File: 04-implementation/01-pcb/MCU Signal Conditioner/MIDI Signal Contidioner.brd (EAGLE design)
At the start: 81.3 x 38.1 mm, 15 parts, among them J2 ARDUINO-CONN-8X2, J3 ARDUINO-CONN-8X2, U4 24CS01, U6 MCP1700-SOT89, X1 SSW-107-02-S-D, X2 SSW-107-02-S-D, X3 SSW-107-02-S-D, X4 SSW-107-02-S-D, X5 MINI-USB-SHIELD-32005-201

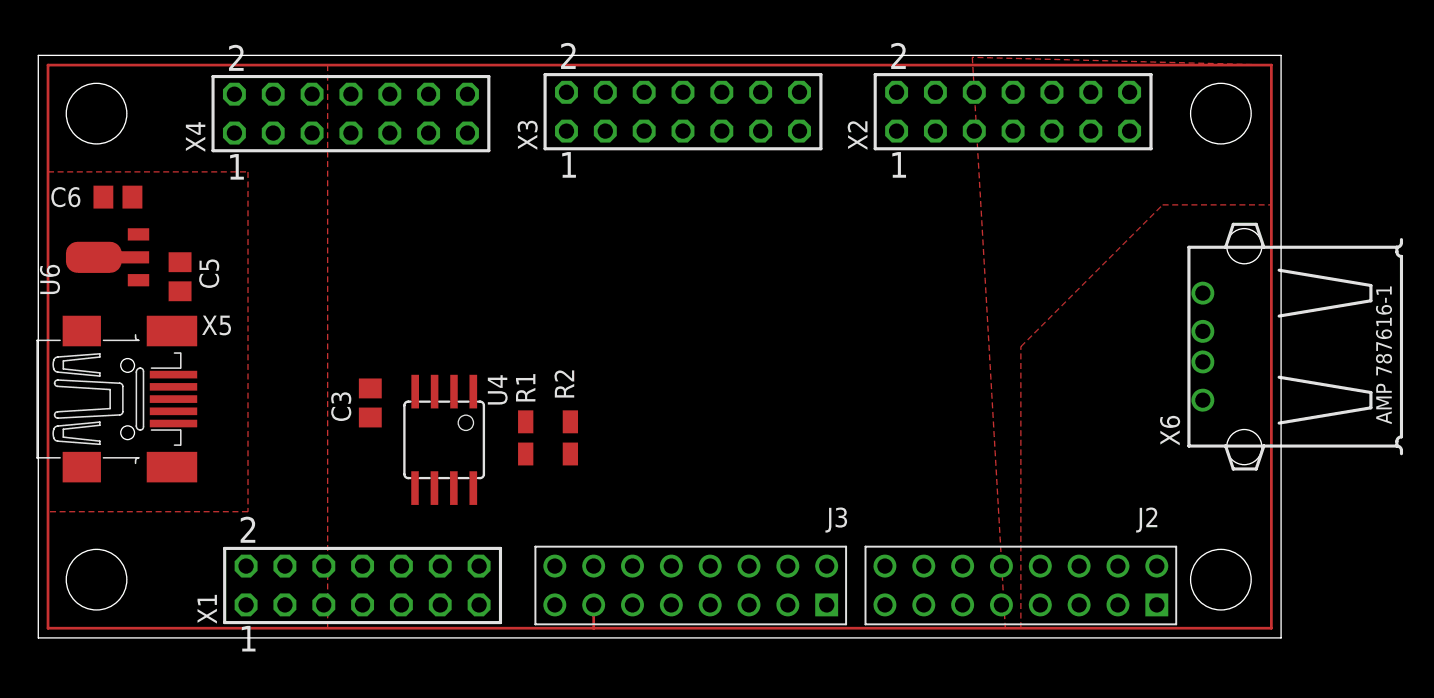
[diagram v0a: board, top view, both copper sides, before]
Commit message: Complete initial placement of components.
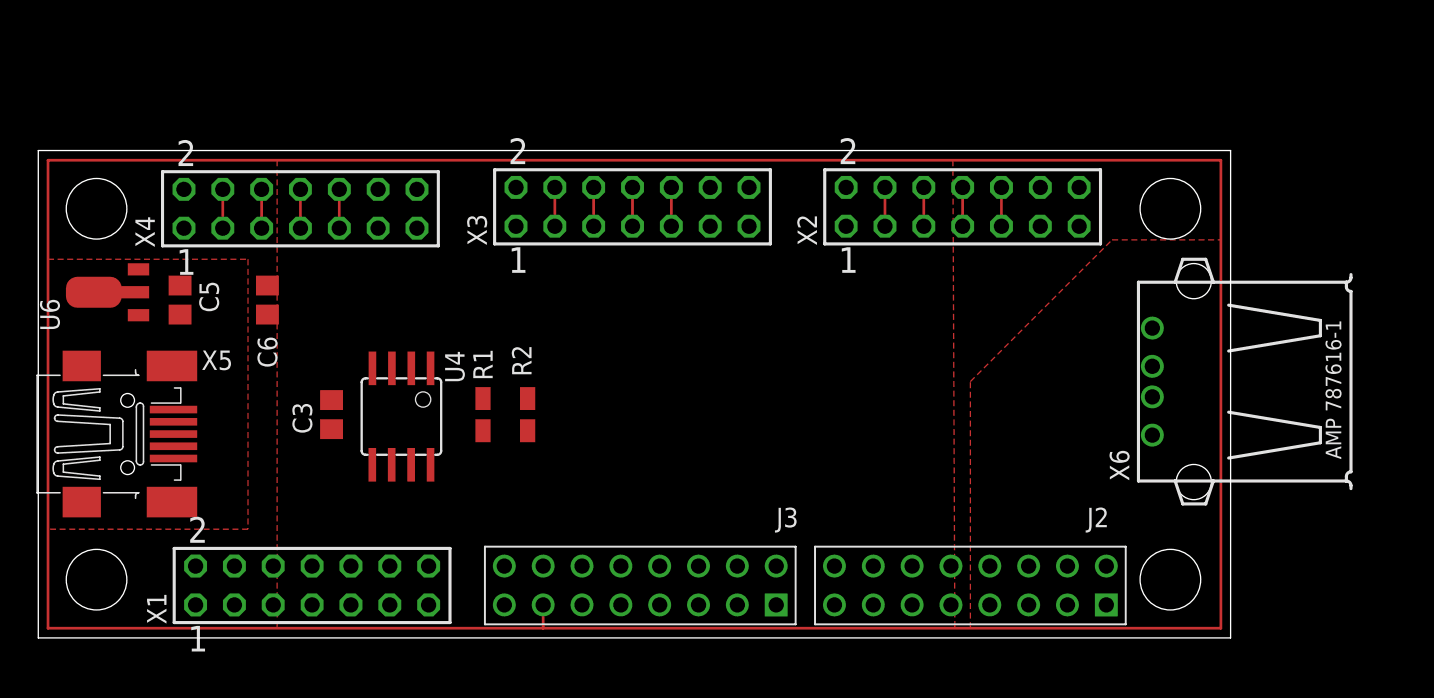
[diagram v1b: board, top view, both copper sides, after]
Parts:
- moved C6 11.9 mm to (15.0, 22.1), turned to 270 degrees
- moved X2 7.04 mm to (60.5, 28.2)
- moved X3 7.04 mm to (38.9, 28.2)
- moved X4 7.04 mm to (17.1, 28.1)
- moved X6 4.02 mm to (85.9, 16.8)
- moved J2 3.30 mm to (69.8, 2.16)
- moved J3 3.30 mm to (48.3, 2.16)
- moved X1 3.30 mm to (17.9, 3.43)
- moved R2 3.18 mm to (32.0, 14.6)
- moved R1 3.18 mm to (29.1, 14.6)
- moved U4 3.18 mm to (23.7, 14.5)
- moved C3 2.65 mm to (19.2, 14.6)
- moved X5 2.29 mm to (5.84, 13.3)
- moved U6 2.29 mm to (4.57, 22.6)
- moved C5 1.52 mm to (9.27, 22.1)
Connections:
- net GND: now also X5.M1, X5.M2, X5.M3, X5.M4
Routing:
- net +5V: track 235.2 -> 216.2 mm
- net DI4: track 0.00 -> 5.08 mm
- net DI3: track 0.00 -> 5.08 mm
- net DI2: track 0.00 -> 5.08 mm
- net DI1: track 0.00 -> 5.08 mm
- net DO4: track 0.00 -> 2.54 mm
- net DO3: track 0.00 -> 2.54 mm
- net DO2: track 0.00 -> 2.54 mm
- net DO1: track 0.00 -> 2.54 mm
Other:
- board size 81.3 x 38.1 mm -> 78 x 31.9 mm
